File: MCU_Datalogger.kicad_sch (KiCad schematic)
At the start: 24 parts, among them U1 ATMEGA328P-AU, U2 DS1337S_, U3 24LC1025, U4 24LC1025, Y1 Crystal, Y2 Crystal

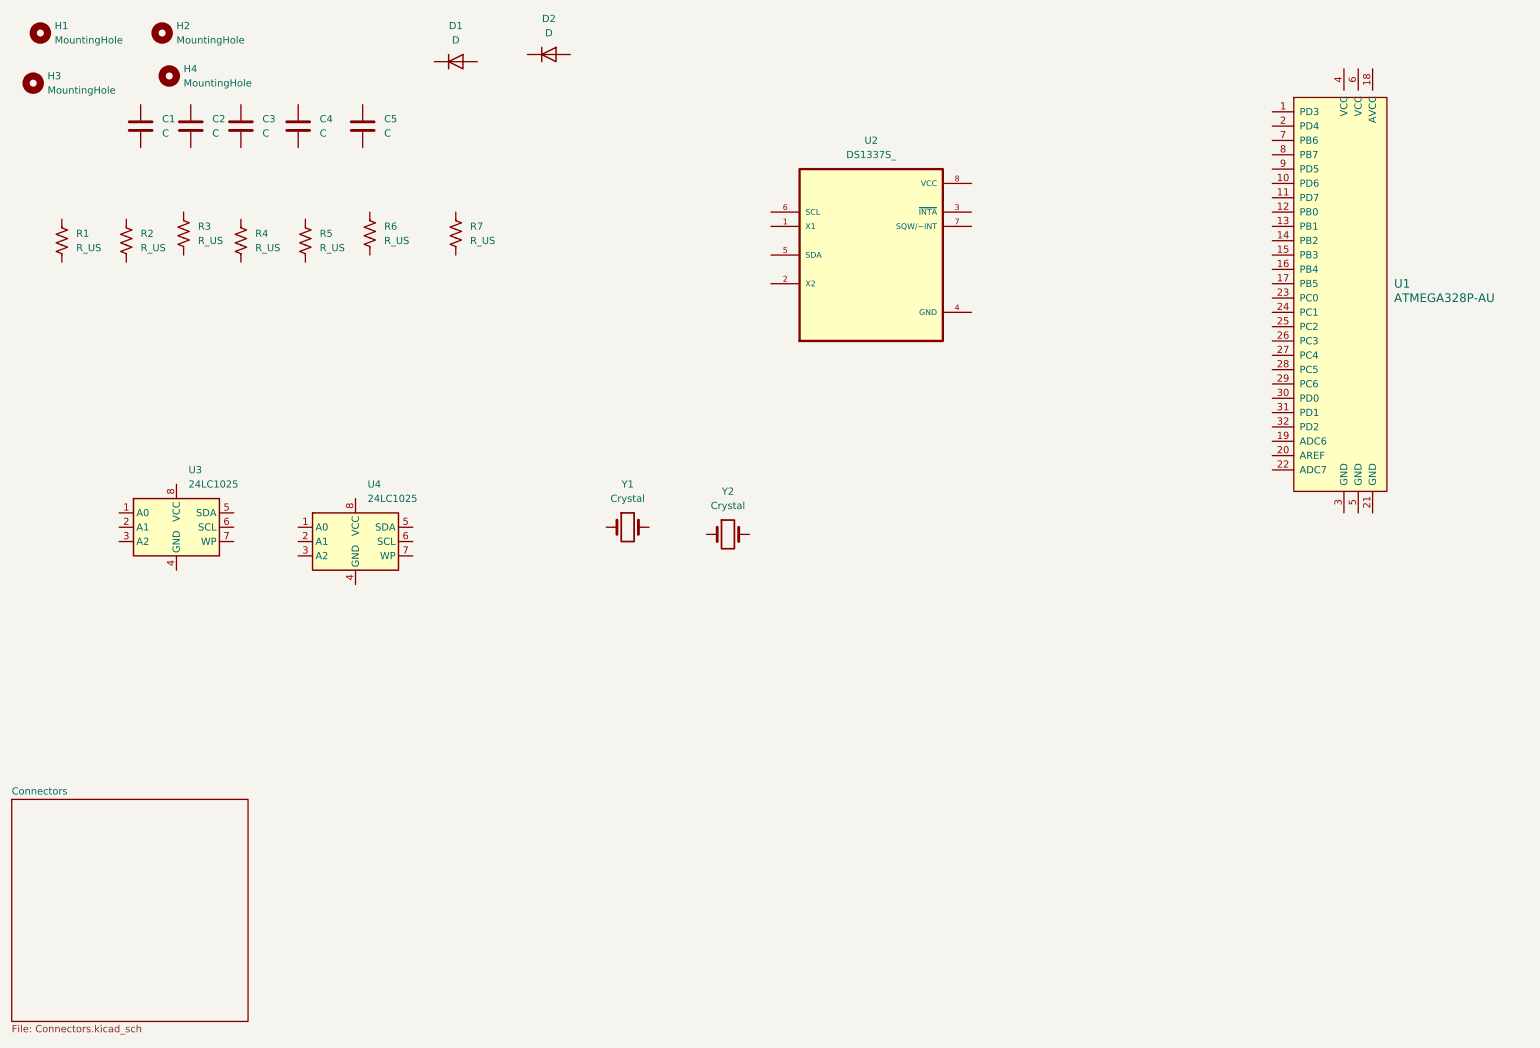
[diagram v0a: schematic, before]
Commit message: Schematic Complete
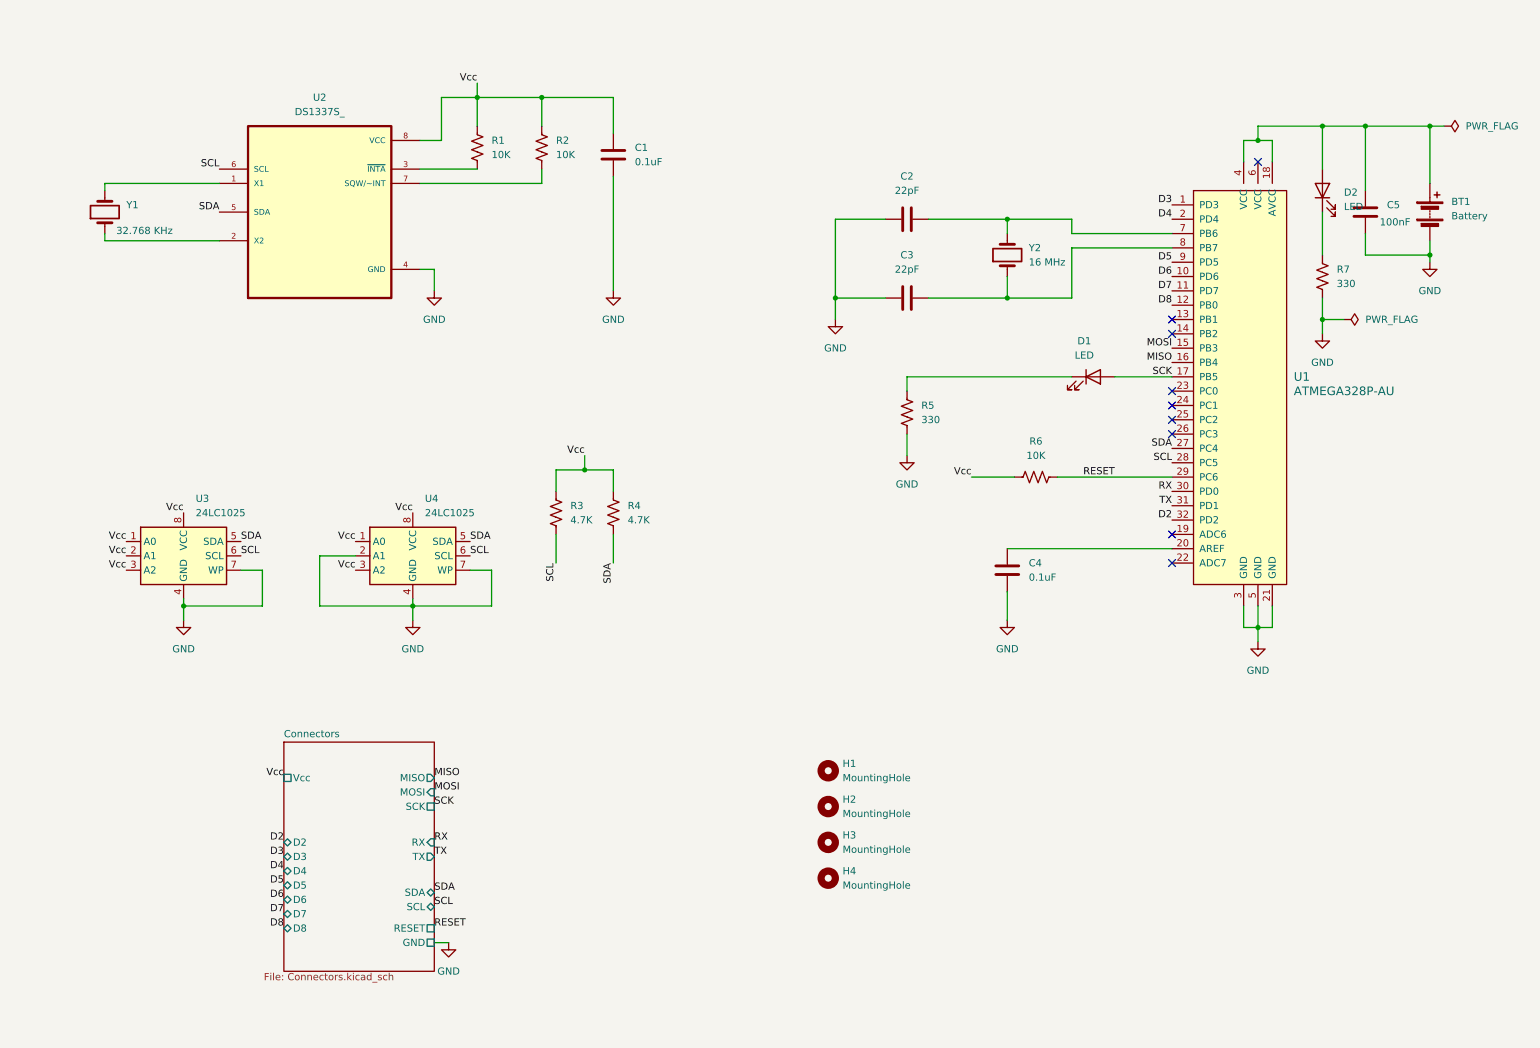
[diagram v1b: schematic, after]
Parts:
- removed D1, D2: D, symbol Device:D
- added BT1: Battery, Connector_PinHeader_2.54mm:PinHeader_1x02_P2.54mm_Vertical, symbol Device:Battery
- added D1, D2: LED, symbol Device:LED
- C1, C4: value C -> 0.1uF; footprint (none) -> Capacitor_SMD:C_0805_2012Metric
- C2, C3: value C -> 22pF; footprint (none) -> Capacitor_SMD:C_0805_2012Metric
- C5: value C -> 100nF; footprint (none) -> Capacitor_SMD:C_0805_2012Metric
- H1, H2, H3, H4: footprint (none) -> MountingHole:MountingHole_2.1mm
- R1, R2, R6: value R_US -> 10K; footprint (none) -> Resistor_SMD:R_0805_2012Metric
- R3, R4: value R_US -> 4.7K; footprint (none) -> Resistor_SMD:R_0805_2012Metric
- R5, R7: value R_US -> 330; footprint (none) -> Resistor_SMD:R_0805_2012Metric
- U3, U4: footprint (none) -> Package_SO:SOIC-8_5.3x5.3mm_P1.27mm
- Y1: value Crystal -> 32.768 KHz; footprint (none) -> Crystal:Crystal_SMD_5032-2Pin_5.0x3.2mm_HandSoldering
- Y2: value Crystal -> 16 MHz; footprint (none) -> Crystal:Crystal_SMD_5032-2Pin_5.0x3.2mm_HandSoldering
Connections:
- net at R7.1: now also D2.1 (K)
- net GND: now reaches R7.2
- net GND: now also C1.2, C2.1, C3.1, C4.2, C5.2, R5.1, U1.21 (GND), U1.3 (GND), U1.5 (GND), U2.4 (GND), U3.4 (GND), U3.7 (WP), U4.2 (A1), U4.4 (GND), U4.7 (WP), BT1.2 (-)
- net at C4.1: now also U1.20 (AREF)
- net at C5.1: now also U1.18 (AVCC), U1.4 (VCC), BT1.1 (+), D2.2 (A)
- net Vcc: now reaches R4.1
- net Vcc: now also C1.1, R1.1, R2.1, R3.1, R6.1, U2.8 (VCC), U3.1 (A0), U3.2 (A1), U3.3 (A2), U3.8 (VCC), U4.1 (A0), U4.3 (A2), U4.8 (VCC)
- net SDA: now reaches R4.2
- net SDA: now also U1.27 (PC4), U2.5 (SDA), U3.5 (SDA), U4.5 (SDA)
- net at R2.2: now also U2.7 (SQW/~INT)
- net at R5.2: now also D1.1 (K)
- net RESET: now reaches R6.2
- net RESET: now also U1.29 (PC6)
- net D3: now reaches U1.1 (PD3)
- net D6: now reaches U1.10 (PD6)
- net D7: now reaches U1.11 (PD7)
- net D8: now reaches U1.12 (PB0)
- net MOSI: now reaches U1.15 (PB3)
- net MISO: now reaches U1.16 (PB4)
- net SCK: now reaches U1.17 (PB5)
- net SCK: now also D1.2 (A)
- net D4: now reaches U1.2 (PD4)
- net SCL: now reaches U1.28 (PC5)
- net SCL: now also R3.2, U2.6 (SCL), U3.6 (SCL), U4.6 (SCL)
- net RX: now reaches U1.30 (PD0)
- net TX: now reaches U1.31 (PD1)
- net D2: now reaches U1.32 (PD2)
- net at U1.7 (PB6): now also C2.2, Y2.2
- net at U1.8 (PB7): now also C3.2, Y2.1
- net D5: now reaches U1.9 (PD5)
- net at R1.2: now also U2.3 (~{INTA})
- net at U2.1 (X1): now also Y1.2
- net at U2.2 (X2): now also Y1.1
- no-connect marks 0 -> 9
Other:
- sheet Connectors ports: added D2, D3, D4, D5, D6, D7, D8, GND, MISO, MOSI, RESET, RX, SCK, SCL, SDA, TX, Vcc; removed none
- moved on the sheet: C1, C2, C3, C4, C5, H1, H2, H3, H4, R1, R2, R3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
